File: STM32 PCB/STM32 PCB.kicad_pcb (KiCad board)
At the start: 2 copper layers, 4 parts, among them J1 Screw_Terminal_01x15, J3 Conn_01x08_Pin, U1 NUCLEO-L476RG

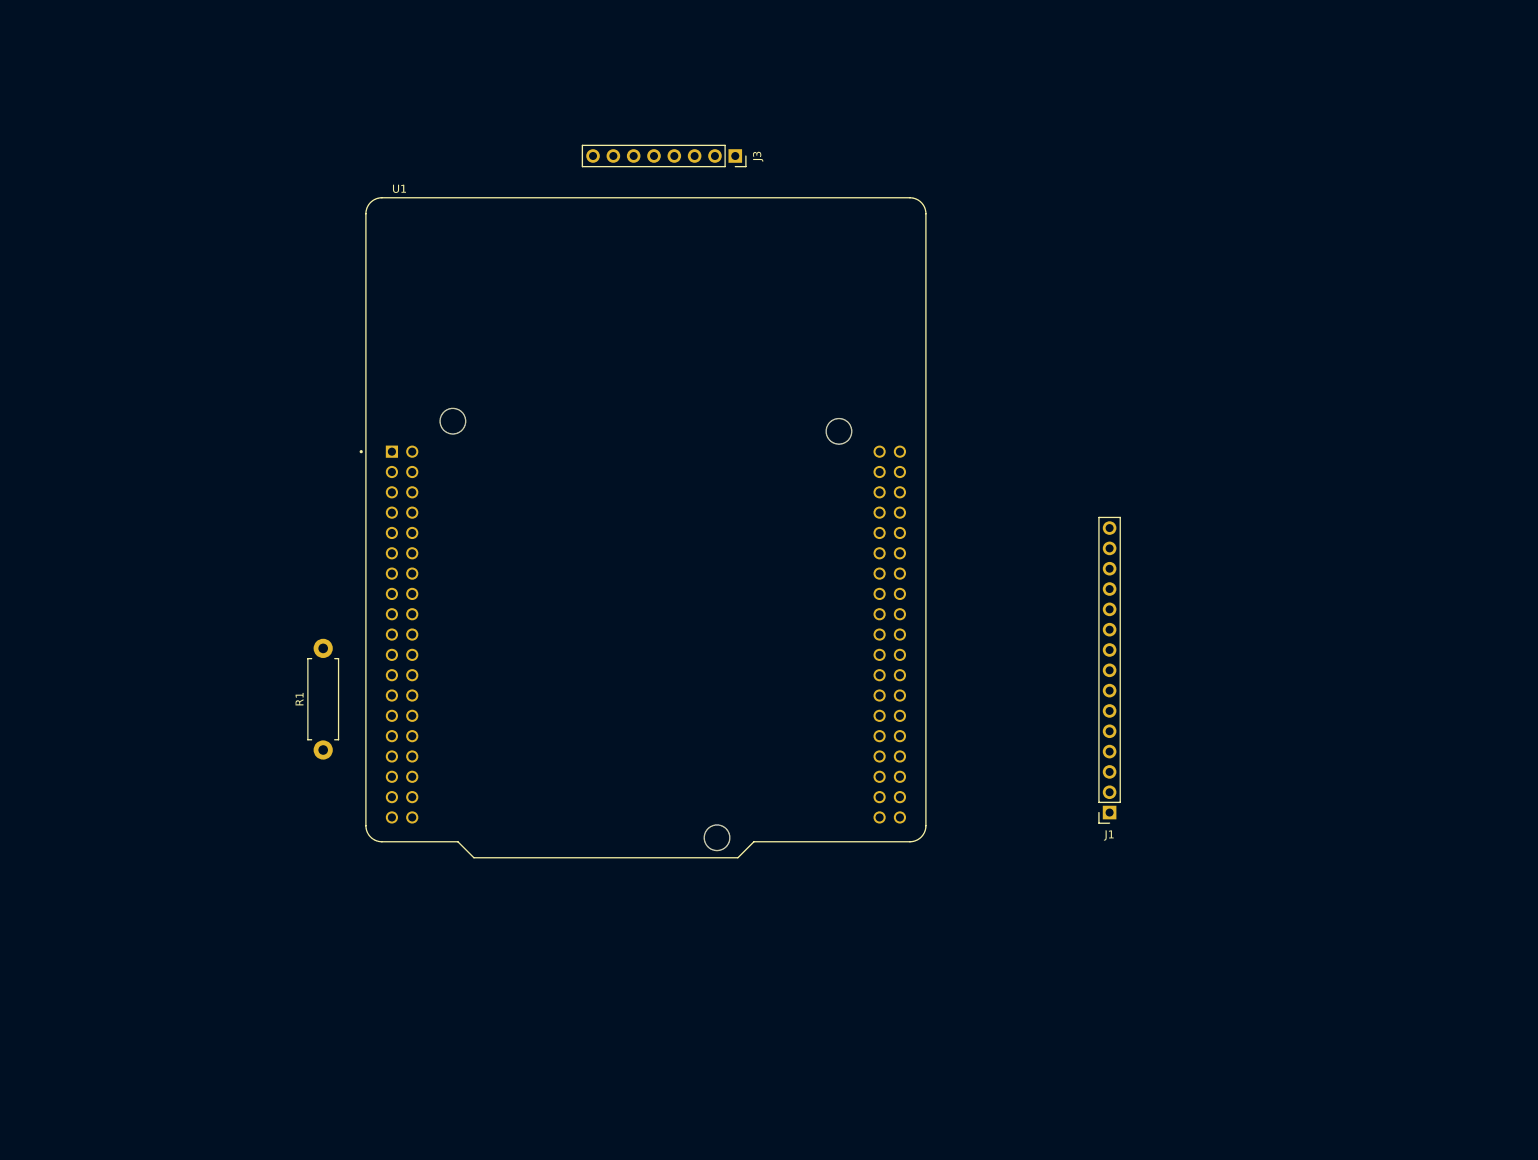
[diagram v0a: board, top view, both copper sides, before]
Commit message: KiCad PCB
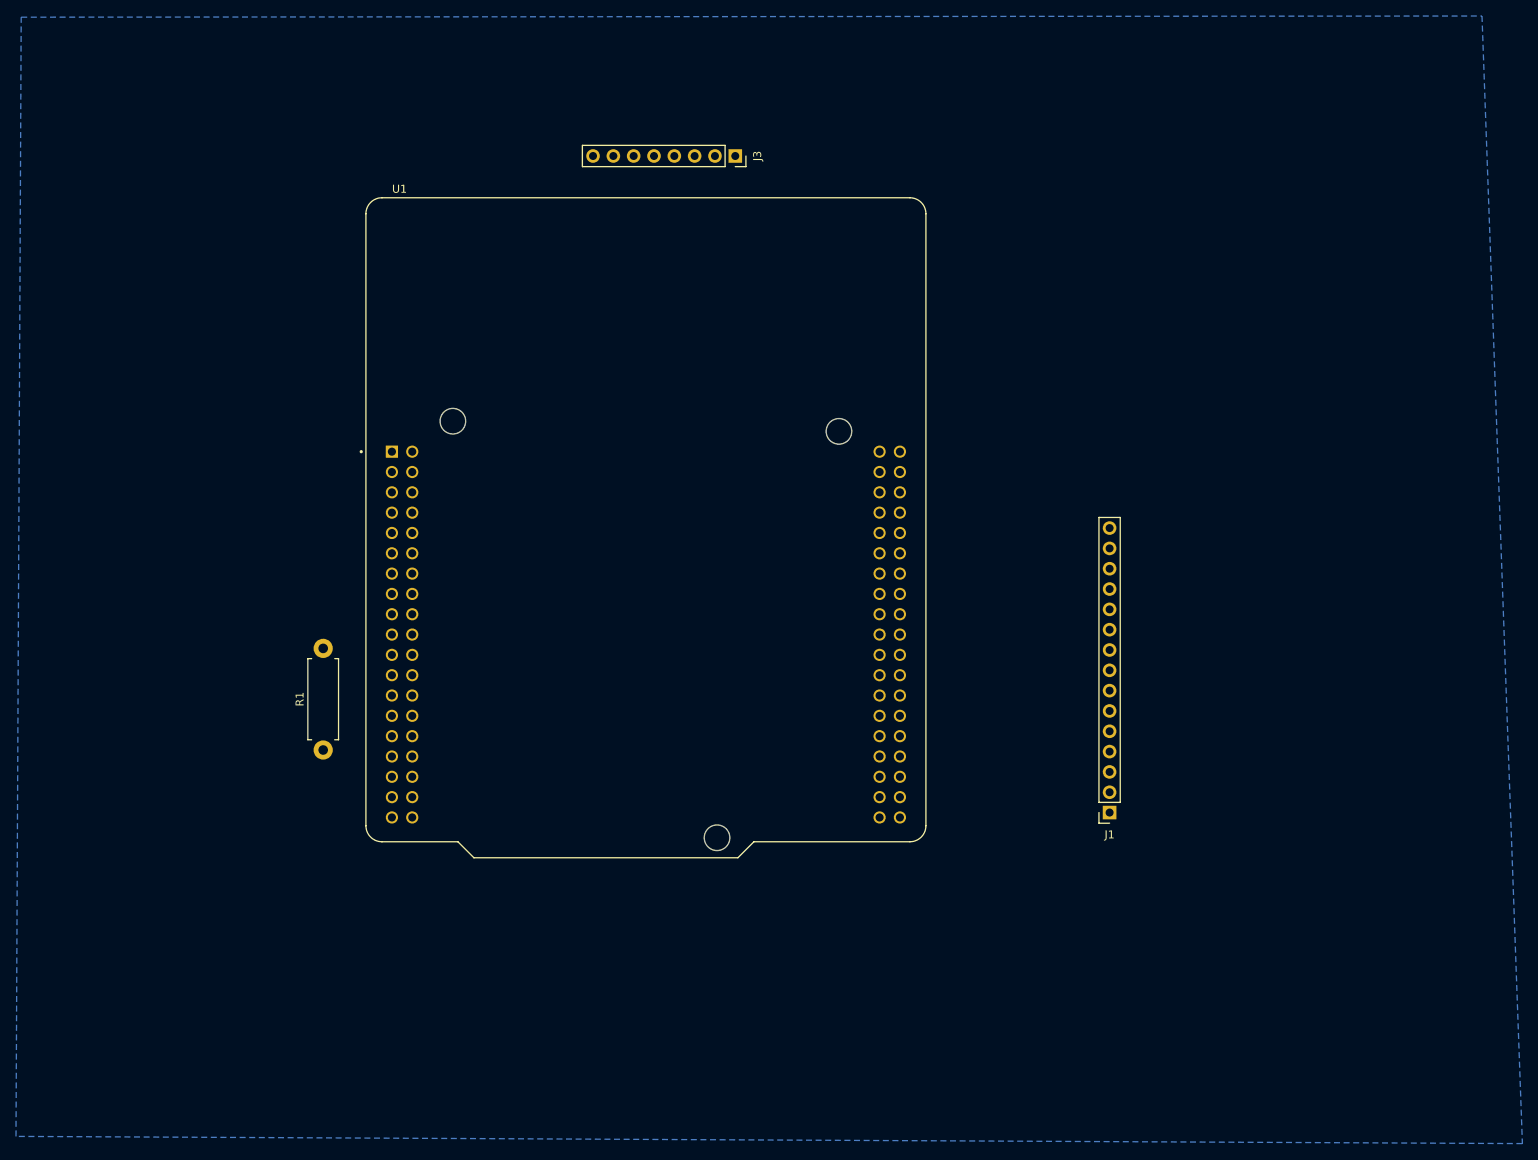
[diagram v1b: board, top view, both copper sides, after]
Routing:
- added copper zone on B.Cu, net GND
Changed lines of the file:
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@@
 	)
 	(setup
+		(stackup
+			(layer "F.SilkS"
+				(type "Top Silk Screen")
+			)
+			(layer "F.Paste"
+				(type "Top Solder Paste")
+			)
+			(layer "F.Mask"
+				(type "Top Solder Mask")
+				(thickness 0.01)
+			)
+			(layer "F.Cu"
+				(type "copper")
+				(thickness 0.035)
+			)
+			(layer "dielectric 1"
+				(type "core")
+				(thickness 1.51)
+				(material "FR4")
+				(epsilon_r 4.5)
+				(loss_tangent 0.02)
+			)
+			(layer "B.Cu"
+				(type "copper")
+				(thickness 0.035)
+			)
+			(layer "B.Mask"
+				(type "Bottom Solder Mask")
+				(thickness 0.01)
+			)
+			(layer "B.Paste"
+				(type "Bottom Solder Paste")
+			)
+			(layer "B.SilkS"
+				(type "Bottom Silk Screen")
+			)
+			(copper_finish "None")
+			(dielectric_constraints no)
+		)
 		(pad_to_mask_clearance 0)
 		(allow_soldermask_bridges_in_footprints no)
@@
 			)
 		)
+	)
+	(zone
+		(net 1)
+		(net_name "GND")
+		(layer "B.Cu")
+		(hatch edge 0.5)
+		(connect_pads
+			(clearance 0.5)
+		)
+		(min_thickness 0.25)
+		(filled_areas_thickness no)
+		(fill
+			(thermal_gap 0.5)
+			(thermal_bridge_width 0.5)
+		)
+		(polygon
+			(pts
+				(xy 89.2 17.35) (xy 271.8 17.2) (xy 276.85 158.15) (xy 88.55 157.25)
+			)
+		)
